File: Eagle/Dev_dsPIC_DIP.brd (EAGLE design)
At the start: 59.4 x 80 mm, 33 parts, among them IC1 DSPIC33FJ64MC802-SP, P1 Vin

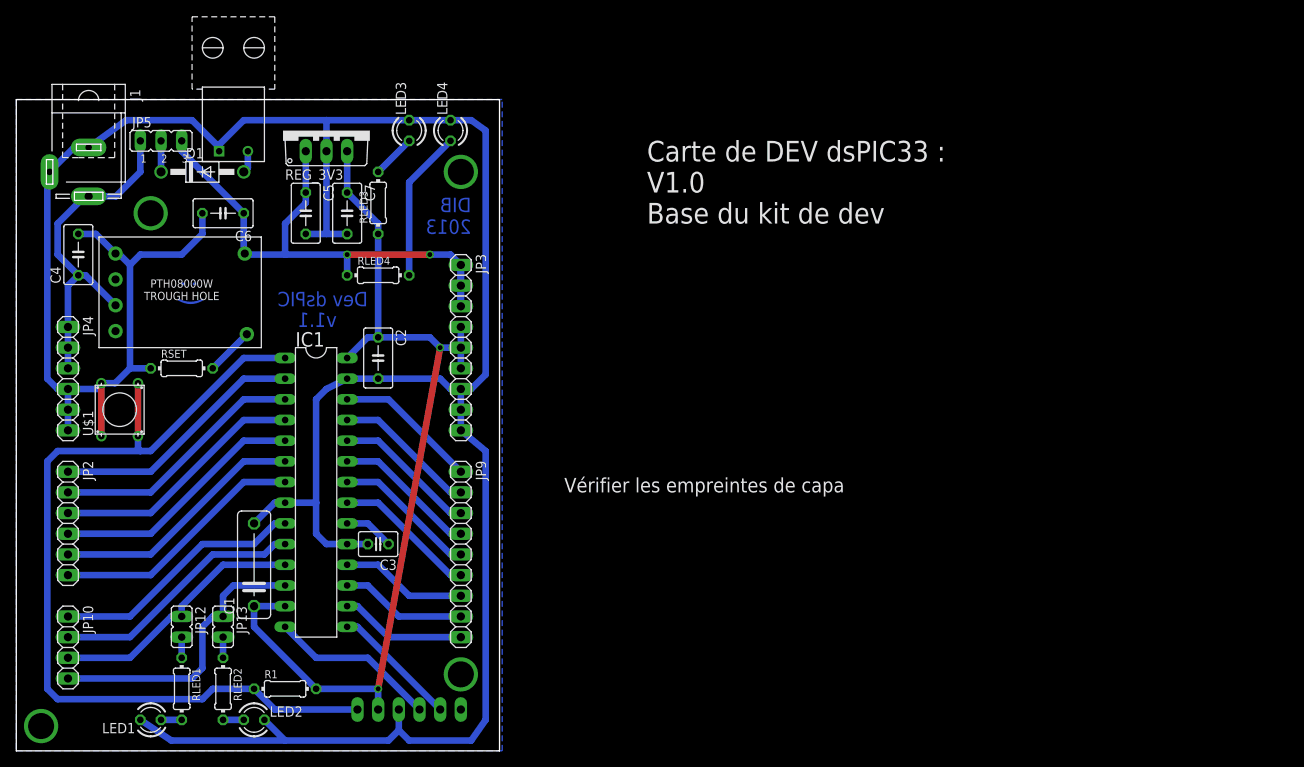
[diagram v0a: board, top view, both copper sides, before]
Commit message: Petit changement au routage et au template
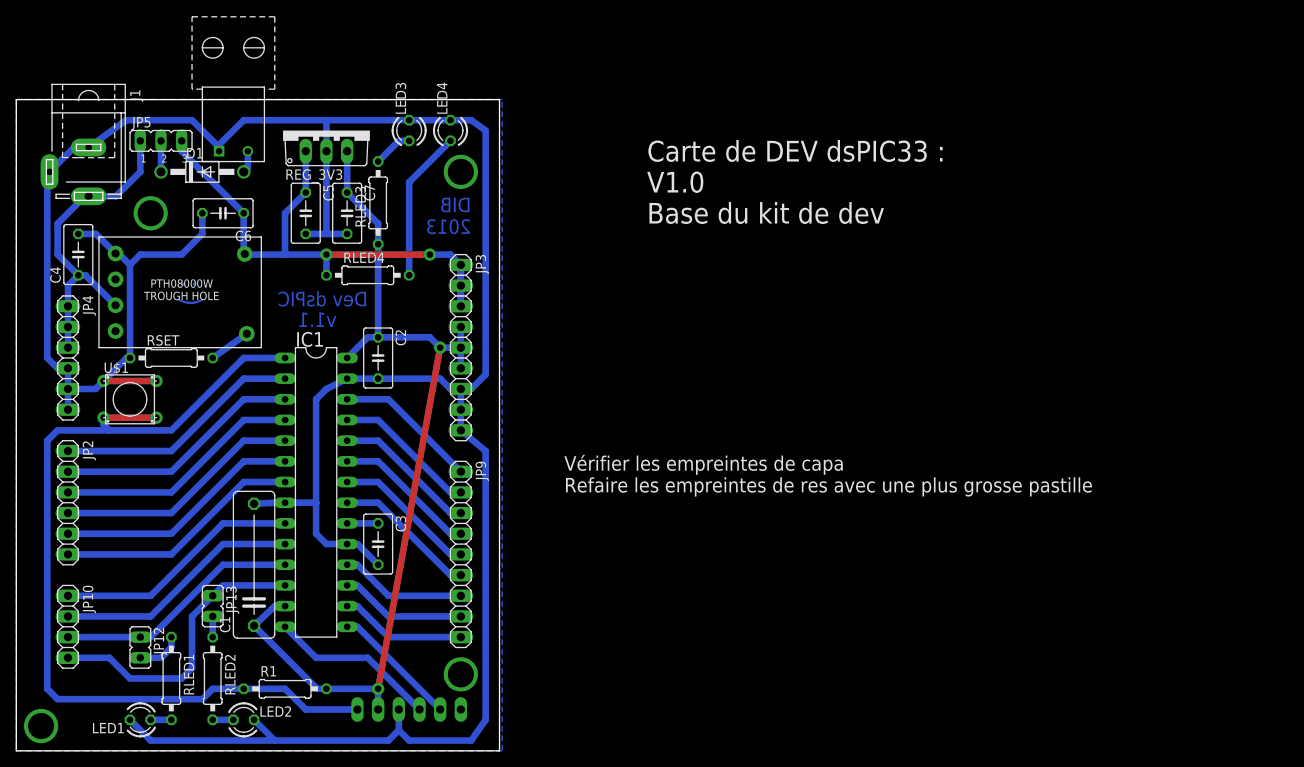
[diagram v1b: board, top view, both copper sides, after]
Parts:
- C1: device rcl:C102-043X133 -> rcl:C150-054X183
- C3: device rcl:C025-030X050 -> rcl:C050-035X075
- IC1: value DSPIC33FJ64MC802-SP -> DSPIC33FJ128MC802-SP
- R1, RLED1, RLED2, RLED3, RLED4, RSET: device rcl:0204/7 -> rcl:0207/10
- moved JP12 5.68 mm to (15.2, 12.7)
- moved JP13 2.84 mm to (24.1, 17.8)
- moved JP10 2.54 mm to (6.35, 15.2)
- moved JP2 2.54 mm to (6.35, 30.5)
- moved JP4 2.54 mm to (6.35, 48.3)
- moved U$1 1.80 mm to (14.0, 43.2), turned to 0 degrees
- moved RLED1 1.80 mm to (19.1, 8.89)
- moved RLED2 1.80 mm to (24.1, 8.89)
- moved RSET 1.80 mm to (19.1, 48.3)
- moved RLED4 1.27 mm to (43.2, 58.4)
- moved LED1 1.27 mm to (15.2, 3.81)
- moved LED2 1.27 mm to (27.9, 3.81)
- turned C3 to 270 degrees
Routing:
- net PE: track 342.6 -> 339.4 mm
- net N$15: track 2.54 -> 5.61 mm
- net VIN: track 42.1 -> 39.5 mm
- net VCAP: track 6.13 -> 3.81 mm
- net RB4: track 32.1 -> 30.4 mm
- net MCLR: track 111.1 -> 112.5 mm
- net +3V3: track 114.9 -> 113.6 mm
- net AN5: track 31.4 -> 30.4 mm
- net N$10: track 31.4 -> 30.4 mm
- net N$11: track 31.4 -> 30.4 mm
- net AN4: track 31.4 -> 30.4 mm
- net AN3: track 31.4 -> 30.4 mm
- net AN2: track 31.4 -> 30.4 mm
- net AN1: track 31.4 -> 30.4 mm
- net AN0: track 31.4 -> 30.4 mm
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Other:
- board text added: "Vérifier les empreintes de capa Refaire les empreintes de res avec une plus grosse pastille"
- board text removed: "Vérifier les empreintes de capa"
